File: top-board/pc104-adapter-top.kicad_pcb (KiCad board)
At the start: 4 copper layers, 92.8 x 32.6 mm, 13 parts, among them J1 Conn_01x13_Male, J10 SAMTEC-SSW-126-01-G-D, J2 Conn_01x13_Male, J3 Conn_01x13_Male, J4 Conn_01x13_Male, J5 Conn_01x13_Male, J6 Conn_01x13_Male, J7 Conn_01x13_Male, J8 Conn_01x13_Male, J9 SAMTEC-SSW-126-01-G-D

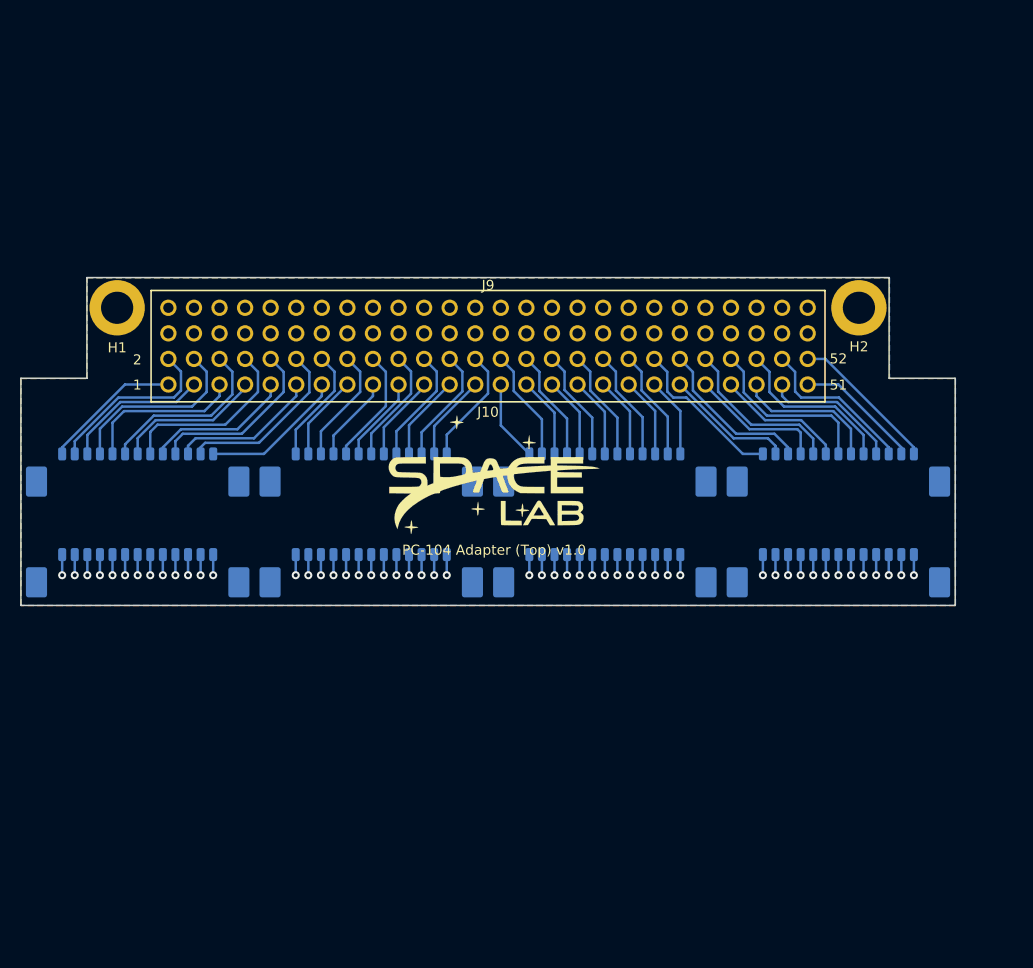
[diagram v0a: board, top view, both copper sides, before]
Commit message: top-board: Version 2.0 #13
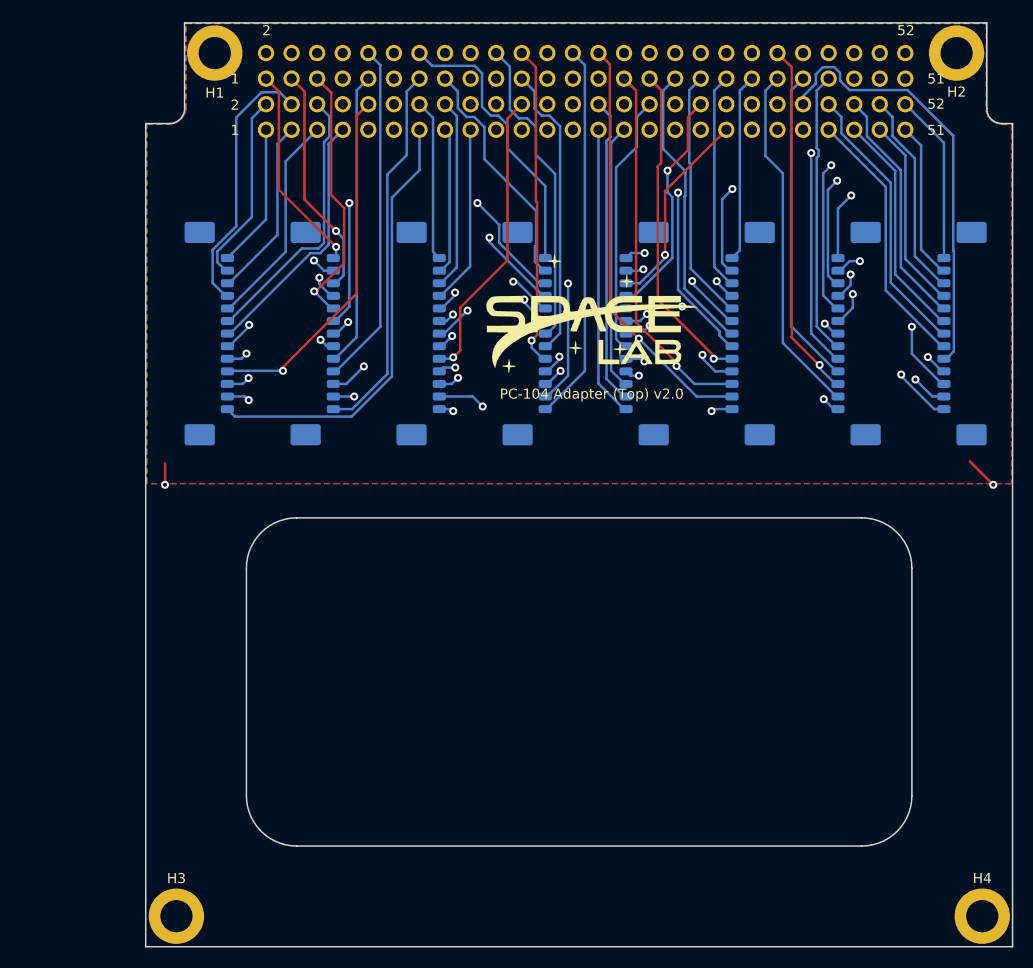
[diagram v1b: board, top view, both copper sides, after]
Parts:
- added H3: MountingHole_Pad, MountingHole:MountingHole_3.2mm_M3_ISO14580_Pad, F.Cu at (105.3, 140.9)
- added H4: MountingHole_Pad, MountingHole:MountingHole_3.2mm_M3_ISO14580_Pad, F.Cu at (185.4, 140.9)
- moved J1 29.5 mm to (119.7, 83.0), turned to 90 degrees
- moved J2 28.2 mm to (140.7, 83.0), turned to 90 degrees
- moved H2 27.1 mm to (182.8, 55.1)
- moved H1 27.1 mm to (109.2, 55.1)
- moved J10 27.1 mm to (146.0, 61.5)
- moved J9 27.1 mm to (146.0, 56.4)
- moved J3 27.0 mm to (161.8, 83.0), turned to 270 degrees
- moved J4 23.2 mm to (172.3, 83.0), turned to 270 degrees
- moved G*** 18.7 mm to (146.6, 81.0)
- moved J8 17.7 mm to (182.8, 83.0), turned to 270 degrees
- moved J5 15.3 mm to (109.2, 83.0), turned to 90 degrees
- moved J6 14.3 mm to (130.2, 83.0), turned to 90 degrees
- moved J7 13.6 mm to (151.3, 83.0), turned to 270 degrees
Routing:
- net GND: track 0.00 -> 92.0 mm, vias 0 -> 2
- net /B13: track 14.3 -> 43.9 mm
- net /B25: track 8.58 -> 36.1 mm, vias 0 -> 1
- net /B44: track 16.7 -> 43.4 mm
- net /B26: track 11.7 -> 36.9 mm, vias 0 -> 1
- net /B40: track 15.8 -> 38.8 mm, vias 0 -> 1
- net /B24: track 11.6 -> 33.1 mm, vias 0 -> 1
- net /B41: track 12.8 -> 34.2 mm, vias 0 -> 1
- net /B23: track 8.57 -> 29.8 mm, vias 0 -> 1
- net /B27: track 8.07 -> 29.0 mm
- net /B12: track 17.6 -> 38.2 mm, vias 0 -> 1
- net /B28: track 11.1 -> 30.6 mm
- net /B42: track 16.1 -> 34.7 mm, vias 0 -> 1
- net /B29: track 8.05 -> 26.5 mm
- net /B30: track 11.1 -> 29.4 mm, vias 0 -> 1
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- added copper zone on F.Cu, net GND
- removed copper zone on F.Cu, net (none)
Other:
- board size 92.8 x 32.6 mm -> 86.1 x 91.8 mm
- board text added: "PC-104 Adapter (Top) v2.0"
- board text removed: "PC-104 Adapter (Top) v1.0"
